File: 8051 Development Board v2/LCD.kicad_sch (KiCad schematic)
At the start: 4 parts, among them J10 LCM-S01602DTR_M, J11 Conn_01x03, J9 Conn_01x08

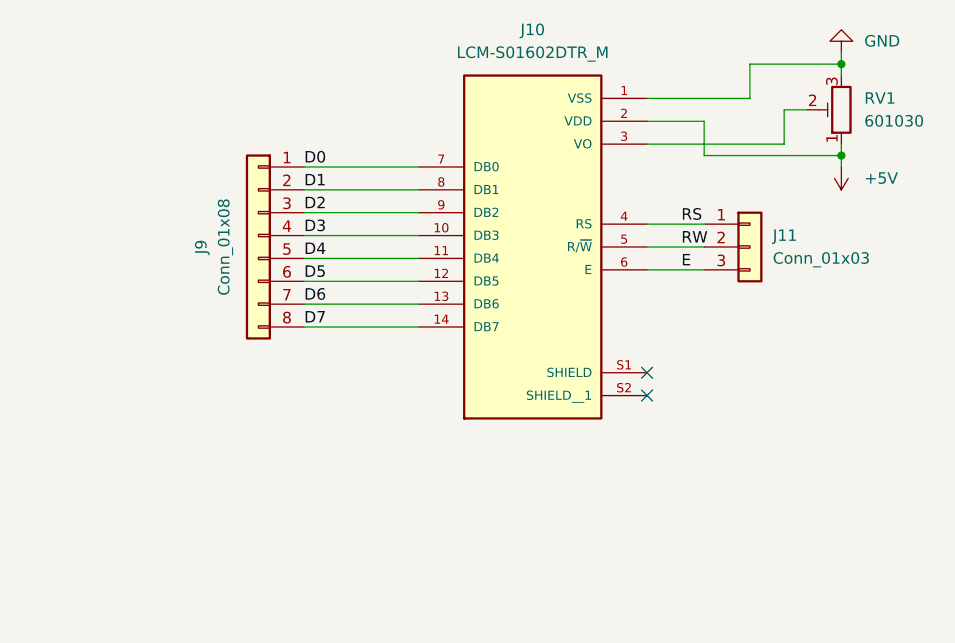
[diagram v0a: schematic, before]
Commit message: ultra
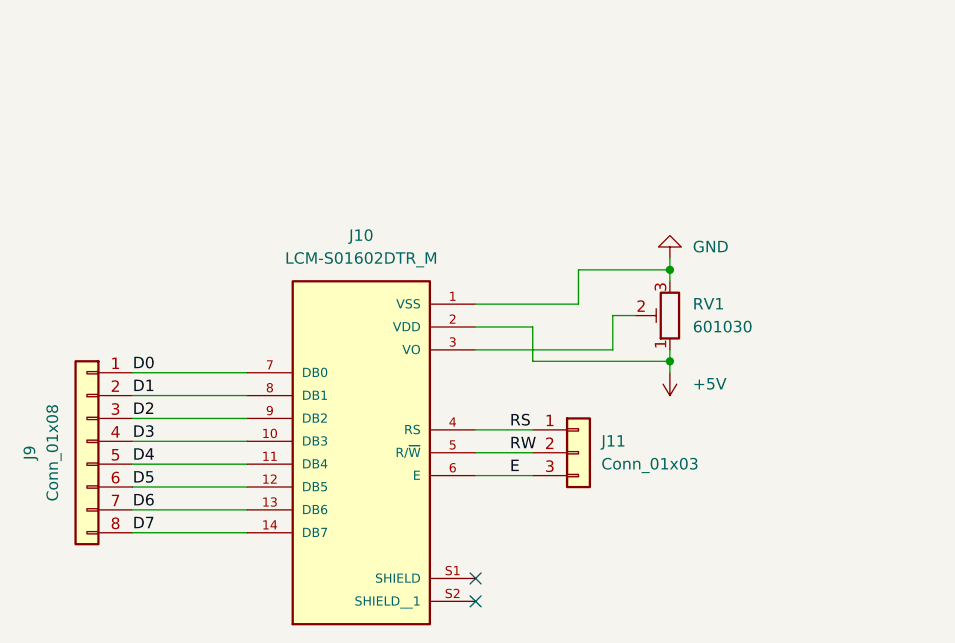
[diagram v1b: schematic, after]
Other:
- moved on the sheet: J10, J11, J9, RV1
